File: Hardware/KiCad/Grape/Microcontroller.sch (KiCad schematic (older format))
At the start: 14 parts, among them U4 ATMEGA328P_TQFP, Y1 16MHz

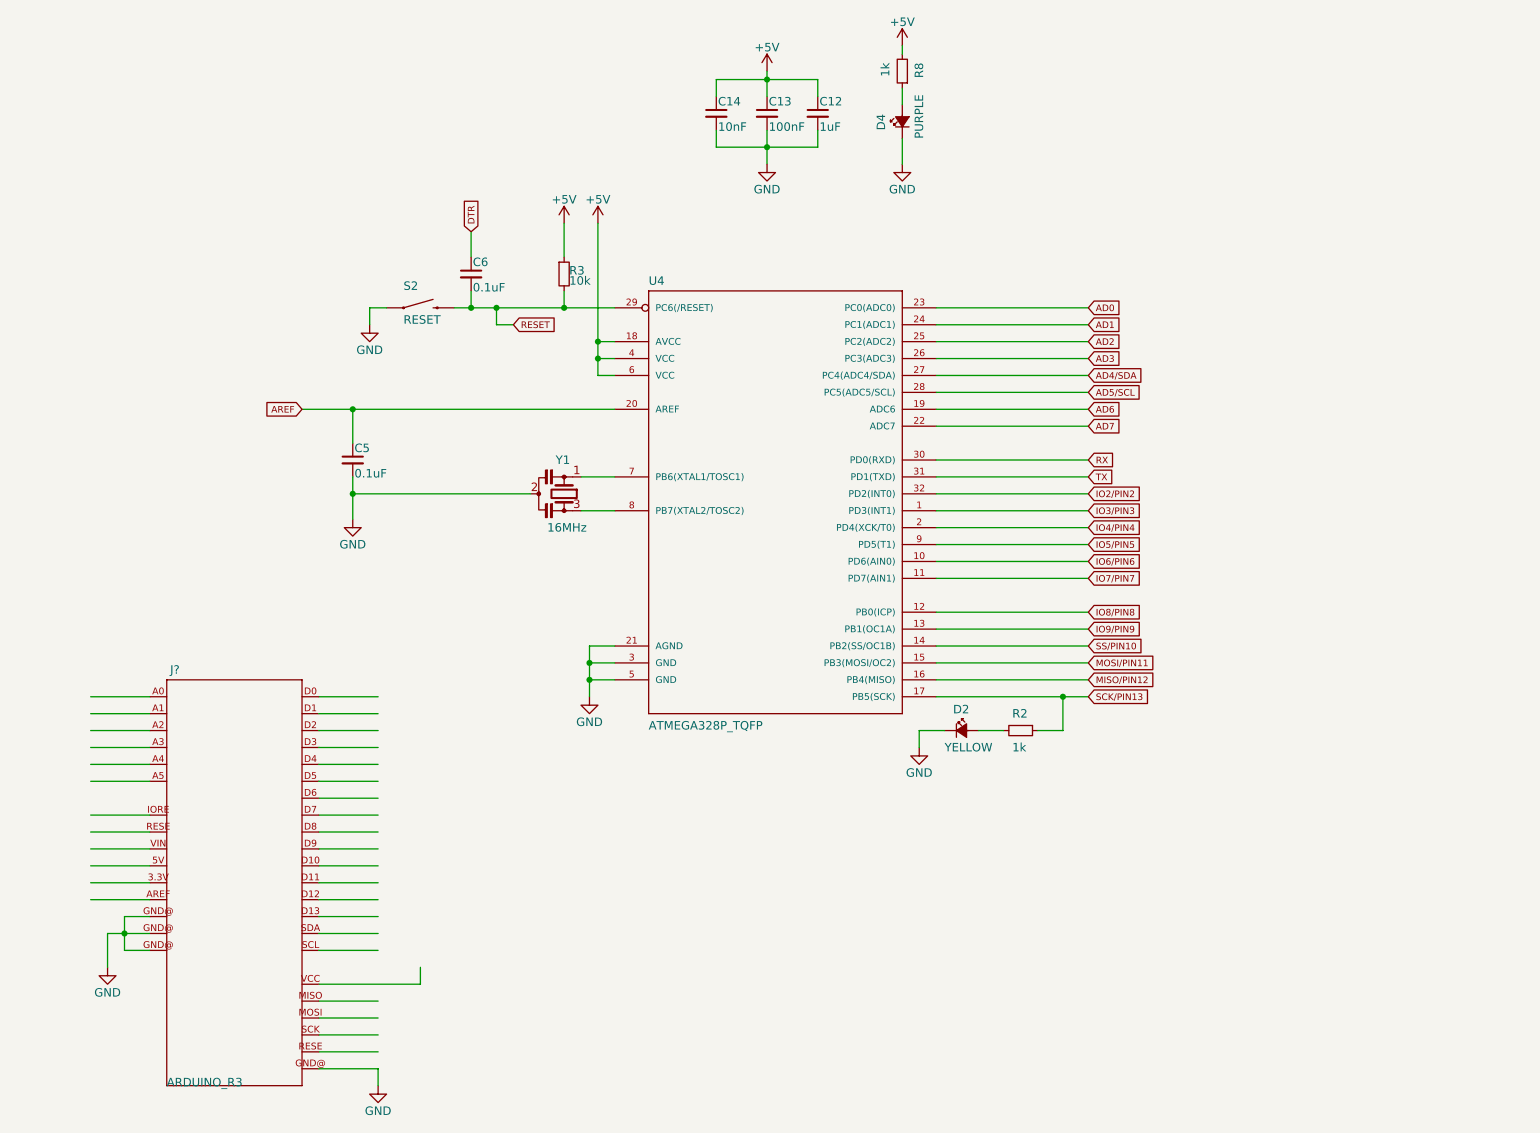
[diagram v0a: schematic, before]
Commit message: Alimentacion comenzada
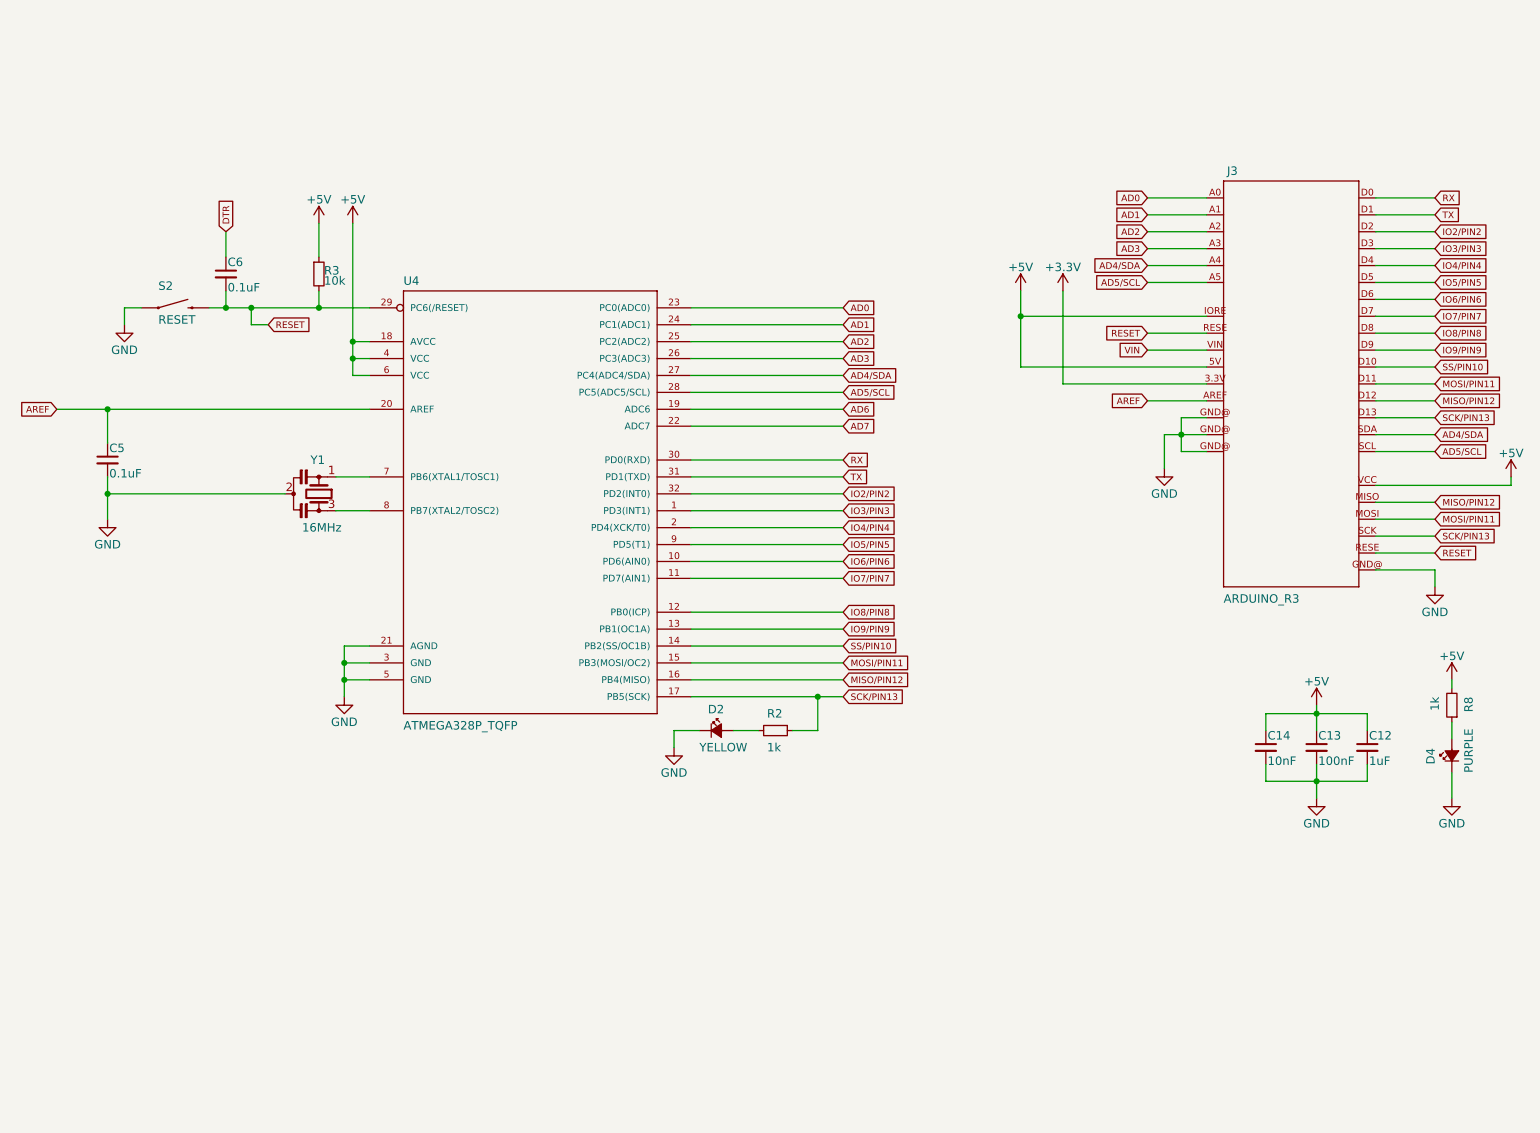
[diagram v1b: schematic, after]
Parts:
- gave numbers to parts that had none: 1
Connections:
- net labels added: +3.3V, VIN
- wire segments 102 -> 104
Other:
- moved on the sheet: C12, C13, C14, C5, C6, D2, D4, J3, R2, R3, R8, S2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
